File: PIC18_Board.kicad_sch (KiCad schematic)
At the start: 1 part, among them U1 PIC18F45K22

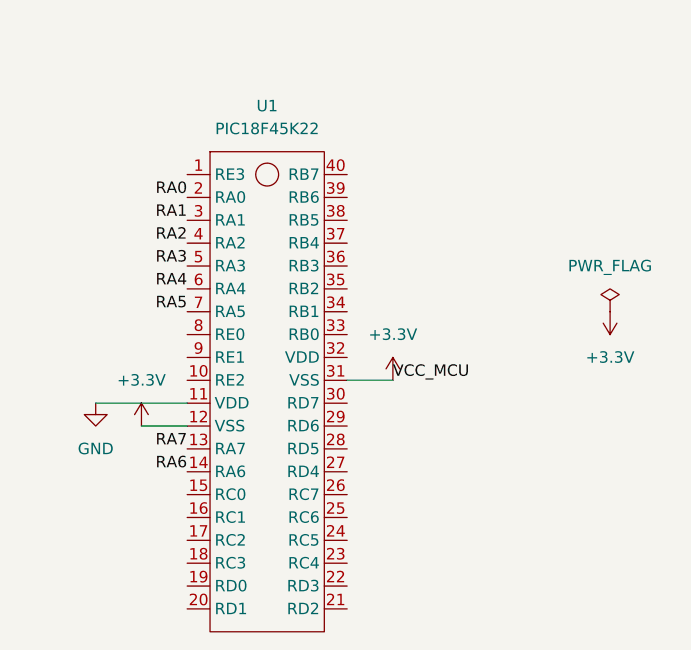
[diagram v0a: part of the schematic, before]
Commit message: Finalized PORTS
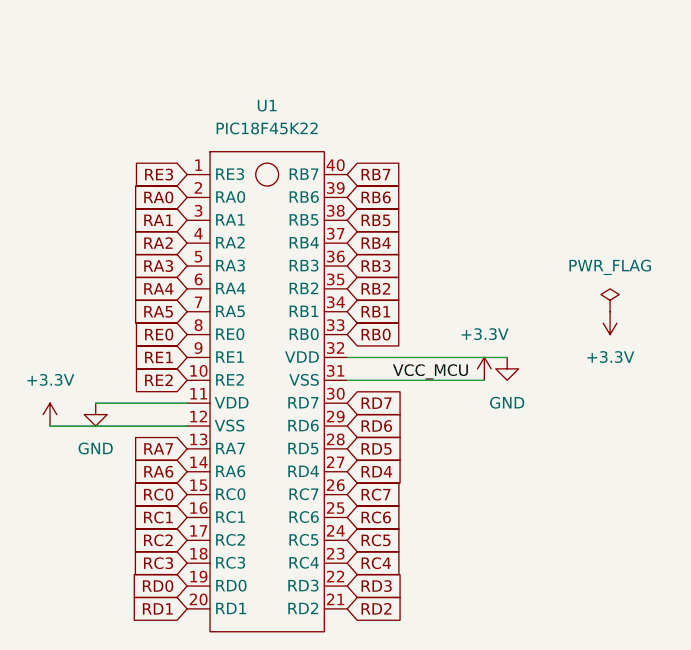
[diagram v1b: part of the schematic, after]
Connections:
- net GND: now also U1.32 (VDD)
- net RE3: now reaches U1.1 (RE3)
- net RE2: now reaches U1.10 (RE2)
- net RC0: now reaches U1.15 (RC0)
- net RC1: now reaches U1.16 (RC1)
- net RC2: now reaches U1.17 (RC2)
- net RC3: now reaches U1.18 (RC3)
- net RD0: now reaches U1.19 (RD0)
- net RD1: now reaches U1.20 (RD1)
- net RD2: now reaches U1.21 (RD2)
- net RD3: now reaches U1.22 (RD3)
- net RC4: now reaches U1.23 (RC4)
- net RC5: now reaches U1.24 (RC5)
- net RC6: now reaches U1.25 (RC6)
- net RC7: now reaches U1.26 (RC7)
- net RD4: now reaches U1.27 (RD4)
- net RD5: now reaches U1.28 (RD5)
- net RD6: now reaches U1.29 (RD6)
- net RD7: now reaches U1.30 (RD7)
- net RB0: now reaches U1.33 (RB0)
- net RB1: now reaches U1.34 (RB1)
- net RB2: now reaches U1.35 (RB2)
- net RB3: now reaches U1.36 (RB3)
- net RB4: now reaches U1.37 (RB4)
- net RB5: now reaches U1.38 (RB5)
- net RB6: now reaches U1.39 (RB6)
- net RB7: now reaches U1.40 (RB7)
- net RE0: now reaches U1.8 (RE0)
- net RE1: now reaches U1.9 (RE1)
